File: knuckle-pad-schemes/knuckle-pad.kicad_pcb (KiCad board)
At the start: 2 copper layers, 127.6 x 115.3 mm, 66 parts, among them SW1 SW_Push, SW10 SW_Push, SW11 SW_Push, SW12 SW_Push, SW13 SW_Push, SW14 SW_Push, SW15 SW_Push, SW16 SW_Push, SW17 SW_Push, SW18 SW_Push, SW19 SW_Push, SW2 SW_Push, SW20 SW_Push, SW21 SW_Push, SW22 SW_Push, SW23 SW_Push, SW24 SW_Push, SW25 SW_Push, SW26 SW_Push, SW27 SW_Push, SW28 SW_Push, SW29 SW_Push, SW3 SW_Push, SW4 SW_Push, SW5 SW_Push, SW6 SW_Push, SW7 SW_Push, SW8 SW_Push, SW9 SW_Push, U1 ProMicro

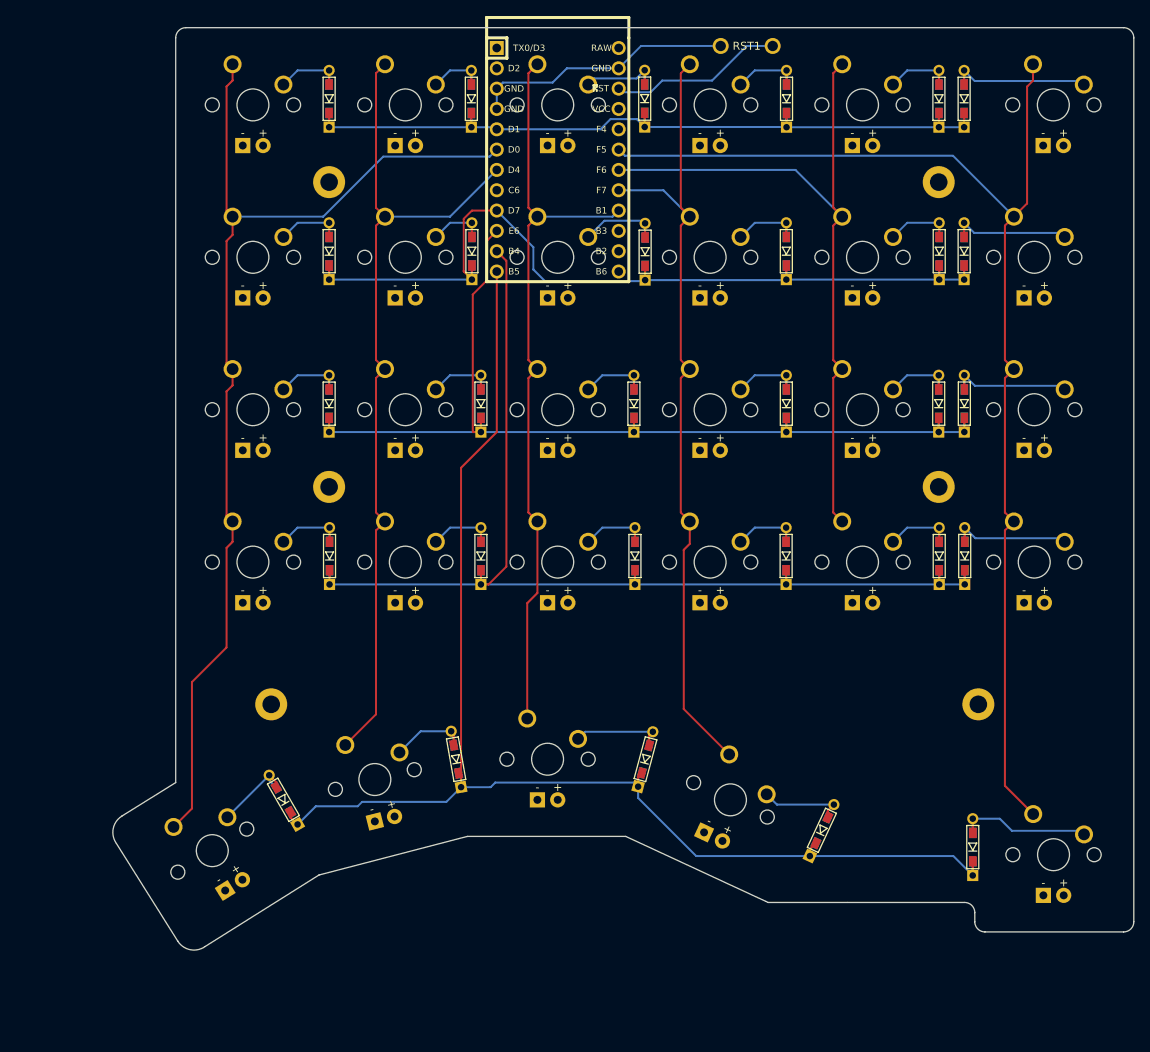
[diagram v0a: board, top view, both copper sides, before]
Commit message: added logo and finalized routing
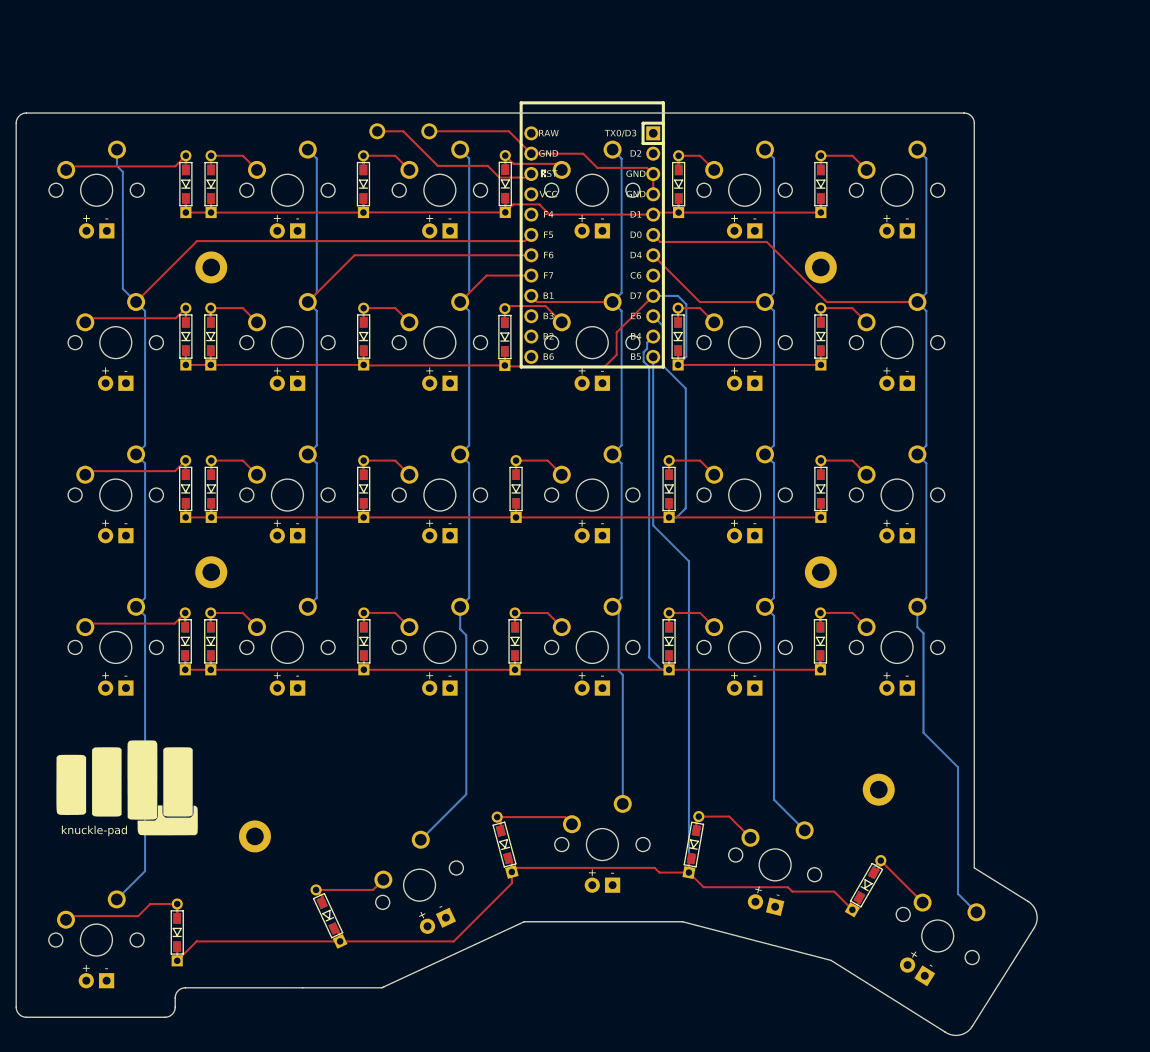
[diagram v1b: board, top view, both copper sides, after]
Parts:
- added G***: LOGO, Hybrid-Switches:logo_fin, F.Cu at (94.7, 118.1)
- D1, D10, D11, D12, D13, D14, D15, D16, D17, D18, D19, D2, D20, D21, D22, D23, D24, D25, D26, D27, D28, D29, D3, D4, D5, D6, D7, D8, D9, RST1, U1: moved to B.Cu
- H1, H2, H3, H4, H5, H6, SW1, SW10, SW11, SW12, SW13, SW14, SW15, SW16, SW17, SW18, SW19, SW2, SW20, SW21, SW22, SW23, SW24, SW25, SW26, SW27, SW28, SW29, SW3, SW4, SW5, SW6, SW7, SW8, SW9: moved to F.Cu
- moved SW5 120.1 mm to (90.9, 137.2), turned to 0 degrees
- moved SW1 120.1 mm to (91.0, 43.4), turned to 0 degrees
- moved SW2 115.3 mm to (93.3, 62.5), turned to 0 degrees
- moved SW3 115.3 mm to (93.3, 81.5), turned to 0 degrees
- moved SW4 115.3 mm to (93.3, 100.6), turned to 0 degrees
- moved D5 100.0 mm to (101.0, 136.2)
- moved D4 98.0 mm to (102.0, 99.8)
- moved D3 97.9 mm to (102.1, 80.8)
- moved D1 97.9 mm to (102.1, 42.7)
- moved D2 97.9 mm to (102.1, 61.7)
- moved H3 91.9 mm to (110.7, 124.2), turned to 0 degrees
- moved D7 91.7 mm to (105.2, 61.7)
- moved D9 91.7 mm to (105.2, 99.8)
- moved D6 91.6 mm to (105.3, 42.7)
- moved D8 91.6 mm to (105.3, 80.8)
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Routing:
- net col5: track 136.8 -> 140.9 mm
- net row2: track 128.1 -> 129.0 mm
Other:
- outline, holes or cut-outs redrawn
- board text added: "knuckle-pad"
